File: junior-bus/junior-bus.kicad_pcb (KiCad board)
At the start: 2 copper layers, 81.3 x 99.1 mm, 4 parts, among them J1 C64AB, J2 C64AC, J3 C64AC, J4 C64AC

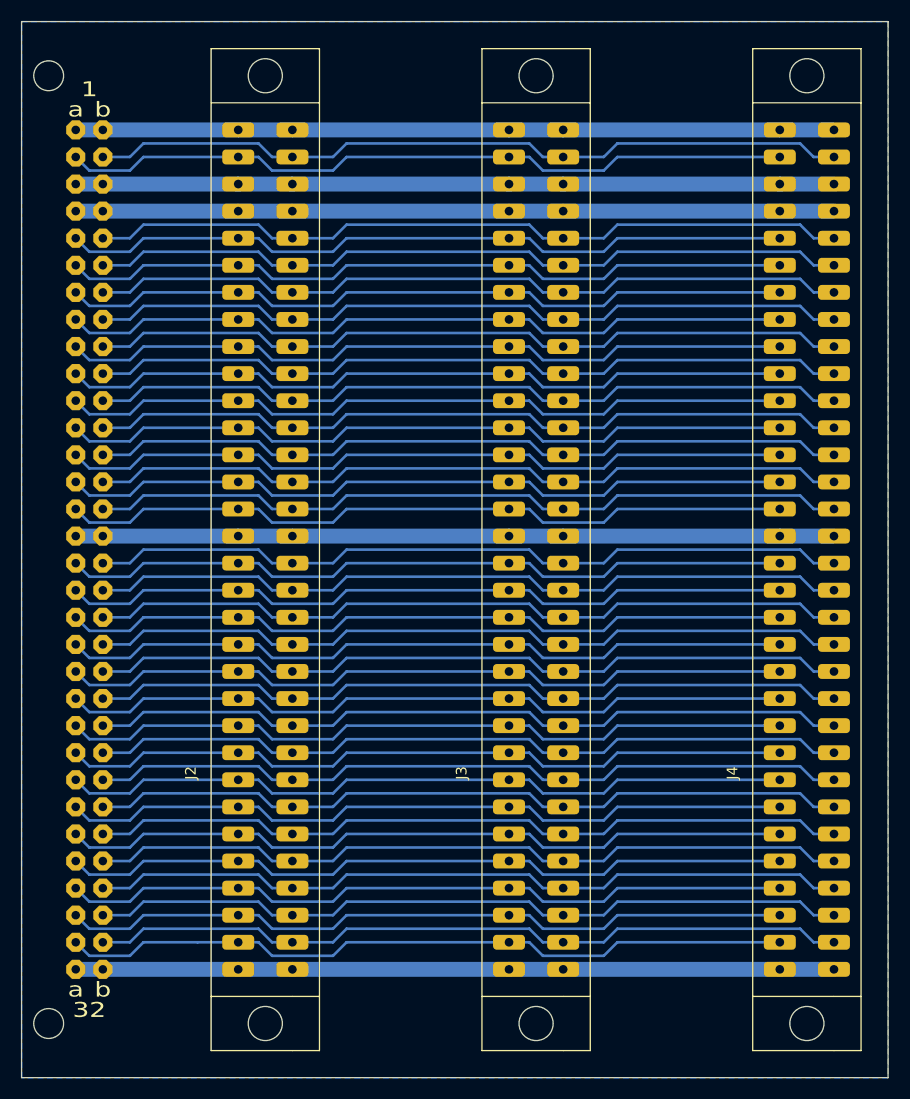
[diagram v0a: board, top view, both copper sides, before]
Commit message: junior ram
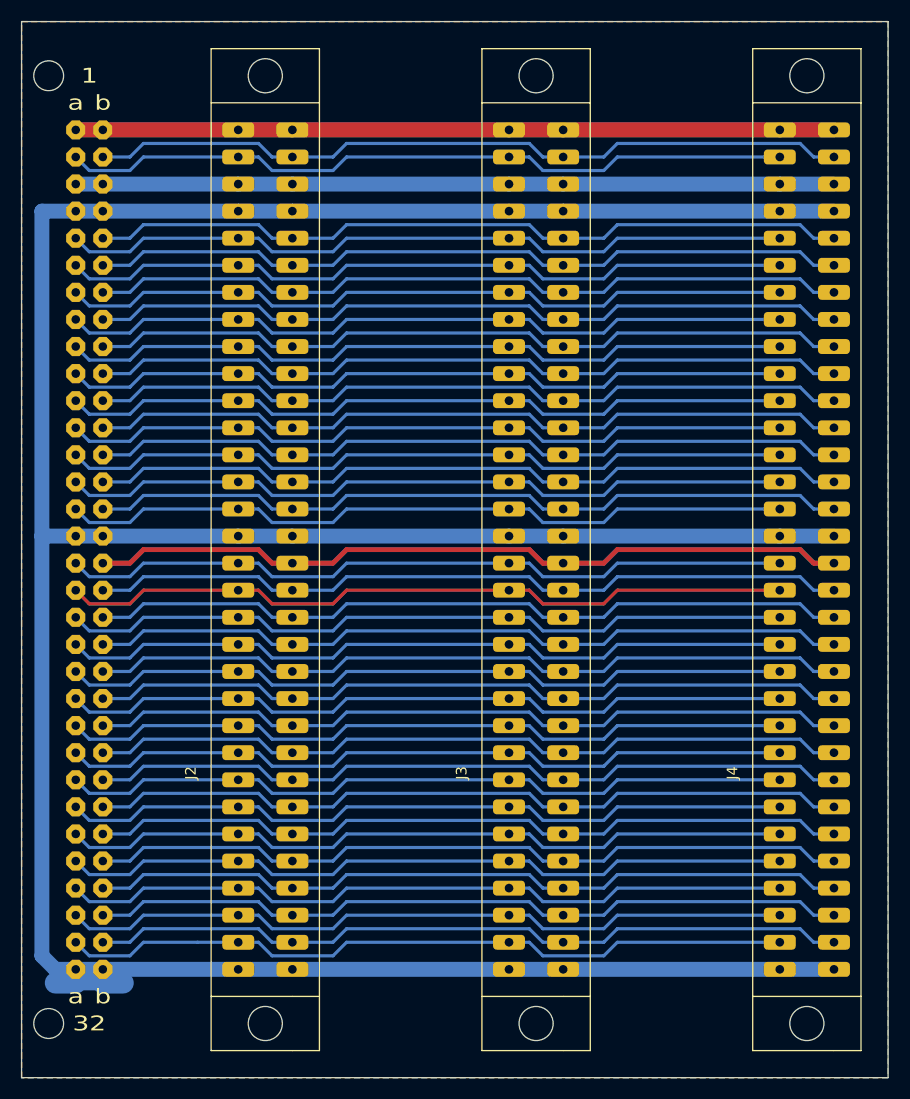
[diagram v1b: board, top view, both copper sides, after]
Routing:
- net GND: track 213.4 -> 302.2 mm
- net +12V: track 71.7 -> 143.5 mm
- net +5V: track 71.1 -> 142.2 mm
- net -5V: track 69.2 -> 138.4 mm
- added copper zone on F.Cu, net GND
